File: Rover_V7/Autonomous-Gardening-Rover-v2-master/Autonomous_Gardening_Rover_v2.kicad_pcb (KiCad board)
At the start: 2 copper layers, 97.5 x 81.7 mm, 42 parts, among them J10 SENSORS, J11 UWB SIGNALS, J13 MOTOR4SIGNAL, J2 USB_B_Micro, J3 Moisture_Power, J4 LINEAR ACTUATOR SIGNAL, J5 MOTOR1SIGNAL, J6 Screw_Terminal_01x02, J7 MOTOR2SIGNAL, J8 Screw_Terminal_01x02, J9 MOTOR3SIGNAL, Q1 SS8050-G, Q2 SS8050-G, SW1 SW_Push, SW2 SW_Push, U1 ESP32-S3-WROOM-1, U2 CP2104

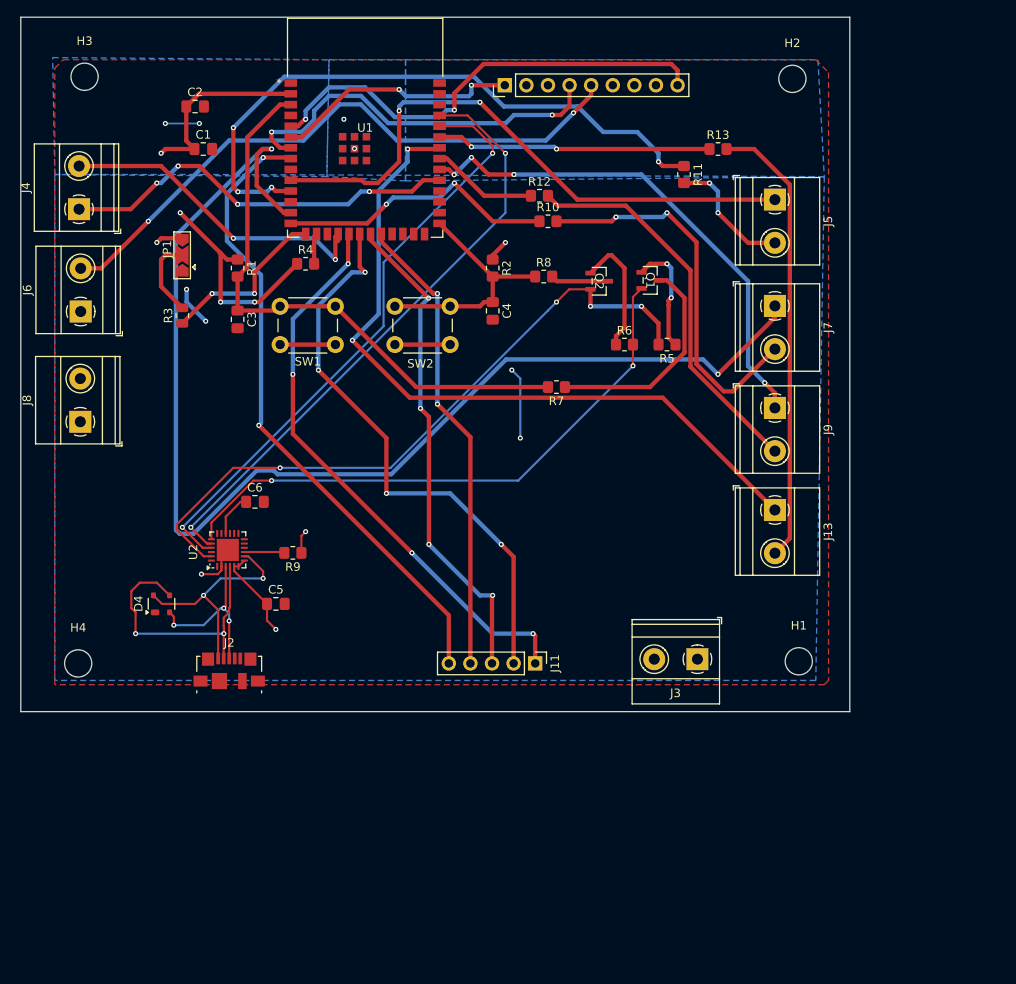
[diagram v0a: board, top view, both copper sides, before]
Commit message: Finish v7 pcb
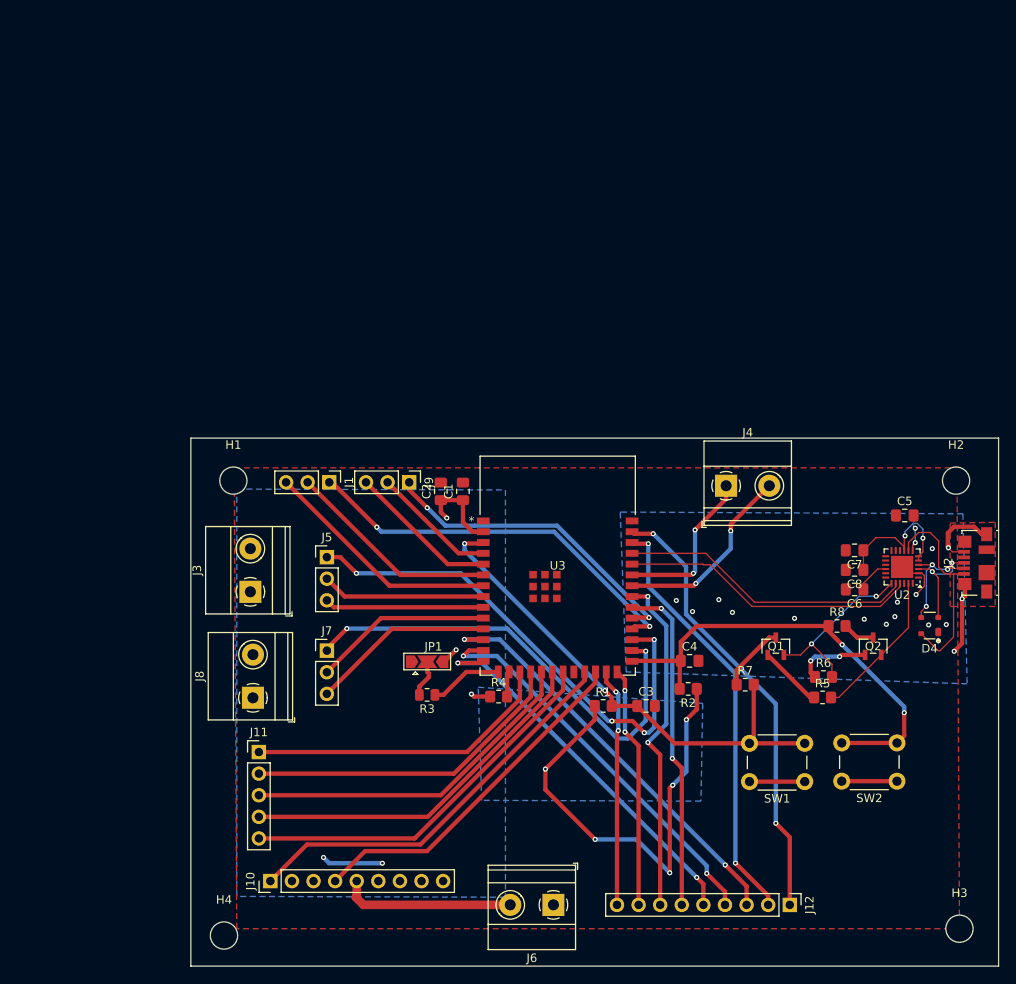
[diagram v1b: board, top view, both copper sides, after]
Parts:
- removed J13: MOTOR4SIGNAL, TerminalBlock_Phoenix:TerminalBlock_Phoenix_MKDS-1,5-2-5.08_1x02_P5.08mm_Horizontal
- removed R10, R11, R12, R13: 5k, Resistor_SMD:R_0805_2012Metric_Pad1.20x1.40mm_HandSolder
- removed R9: 4.7k, Resistor_SMD:R_0805_2012Metric_Pad1.20x1.40mm_HandSolder
- removed U1: ESP32-S3-WROOM-1, ESP32:ESP32-S3-WROOM-1_EXP
- added C7: 1-5uF, Capacitor_SMD:C_0805_2012Metric_Pad1.18x1.45mm_HandSolder, F.Cu at (128.1, 88.2)
- added C8: 0.1uF, Capacitor_SMD:C_0805_2012Metric_Pad1.18x1.45mm_HandSolder, F.Cu at (128.1, 90.5)
- added J1: Conn_01x03_Pin, Connector_PinHeader_2.54mm:PinHeader_1x03_P2.54mm_Vertical, F.Cu at (66.3, 80.2)
- added J12: Conn_01x09_Pin, Connector_PinHeader_2.54mm:PinHeader_1x09_P2.54mm_Vertical, F.Cu at (120.4, 129.9)
- added U3: ESP32-S3-WROOM-1-N16R8, ESP32 S3 WROOM 1 N16R8:ESP32-S3-WROOM-1_EXP, F.Cu at (93.1, 90.0)
- C2: value 100 uF -> 100 n
- C5: value 10uF -> 1uF
- J5: value MOTOR1SIGNAL -> Conn_01x03_Pin; footprint TerminalBlock_Phoenix:TerminalBlock_Phoenix_MKDS-1,5-2-5.08_1x02_P5.08mm_Horizontal -> Connector_PinHeader_2.54mm:PinHeader_1x03_P2.54mm_Vertical
- J7: value MOTOR2SIGNAL -> Conn_01x03_Pin; footprint TerminalBlock_Phoenix:TerminalBlock_Phoenix_MKDS-1,5-2-5.08_1x02_P5.08mm_Horizontal -> Connector_PinHeader_2.54mm:PinHeader_1x03_P2.54mm_Vertical
- J9: value MOTOR3SIGNAL -> Conn_01x03_Pin; footprint TerminalBlock_Phoenix:TerminalBlock_Phoenix_MKDS-1,5-2-5.08_1x02_P5.08mm_Horizontal -> Connector_PinHeader_2.54mm:PinHeader_1x03_P2.54mm_Vertical
- moved H3 143.6 mm to (140.4, 132.7)
- moved J10 97.6 mm to (59.4, 127.1)
- moved D4 90.4 mm to (136.9, 97.0), turned to 180 degrees
- moved J6 89.2 mm to (92.6, 129.9), turned to 180 degrees
- moved J2 88.8 mm to (142.4, 89.7), turned to 90 degrees
- moved J4 82.8 mm to (113.0, 80.6), turned to 0 degrees
- moved U2 79.3 mm to (133.7, 90.2), turned to 180 degrees
- moved SW1 75.4 mm to (122.2, 115.4)
- moved C5 74.7 mm to (134.0, 84.1)
- moved SW2 73.5 mm to (133.1, 115.3)
- moved C6 71.3 mm to (128.1, 92.8), turned to 180 degrees
- moved H1 69.8 mm to (55.0, 80.0)
- moved J5 67.4 mm to (66.0, 89.0), turned to 0 degrees
- moved R1 67.1 mm to (98.5, 106.5), turned to 0 degrees
- moved J7 66.5 mm to (66.0, 100.0), turned to 0 degrees
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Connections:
- C5 pad 1: +3V3 -> VBUS
- C5 pad 2: GND -> Net-(U2-REGIN)
- J5 pad 1: /MOTOR1PWM -> /MOTOR3PWM
- J5 pad 2: /MOTOR1FG -> /MOTOR3ENA
- J7 pad 1: /MOTOR2PWM -> /MOTOR4PWM
- J7 pad 2: /MOTOR2FG -> /MOTOR4ENA
- J9 pad 1: /MOTOR3PWM -> /MOTOR1PWM
- J9 pad 2: /MOTOR3FG -> /MOTOR1ENA
- U2 pad 5: +3V3 -> Net-(U2-VDD)
- U2 pad 6: +3V3 -> Net-(U2-VDD)
- U2 pad 7: +3V3 -> Net-(U2-REGIN)
- U2 pad 9: Net-(U2-~{RST}) -> Net-(U2-VDD)
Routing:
- net /MOTOR2PWM: track 145.4 -> 46.9 mm
- net Net-(U1-IO18): track 74.8 -> 0.00 mm, vias 4 -> 0
- net /DTR: track 79.4 -> 17.7 mm, vias 4 -> 0
- net /Moisture_Sensor_Output: track 55.2 -> 0.00 mm, vias 2 -> 0
- net /MOTOR4FG: track 53.2 -> 0.00 mm
- net /GPIO1: track 0.00 -> 52.9 mm, vias 0 -> 2
- net +5V: track 73.2 -> 20.5 mm, vias 2 -> 0
- net /GPIO2: track 0.00 -> 50.3 mm, vias 0 -> 2
- net /GPIO8: track 0.00 -> 49.6 mm, vias 0 -> 2
- net /RTS: track 69.2 -> 21.0 mm
- net /GPIO19: track 0.00 -> 46.9 mm, vias 0 -> 2
- net /MOTOR3FG: track 45.8 -> 0.00 mm
- net /MOTOR2FG: track 45.3 -> 0.00 mm, vias 2 -> 0
- net /GPIO20: track 0.00 -> 45.2 mm, vias 0 -> 2
- net /GPIO40: track 0.00 -> 40.5 mm, vias 0 -> 2
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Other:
- board size 97.5 x 81.7 mm -> 95 x 62.1 mm
